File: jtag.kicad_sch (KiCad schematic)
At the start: 50 parts, among them J3 USB_C_Receptacle, J4 Conn_01x02_Male, J5 3220-10-0100-00, U10 NTB0104BQ,115, U13 NTB0104BQ,115, U17 93C56, U2 FT2232HL-REEL, Y2 12MHz

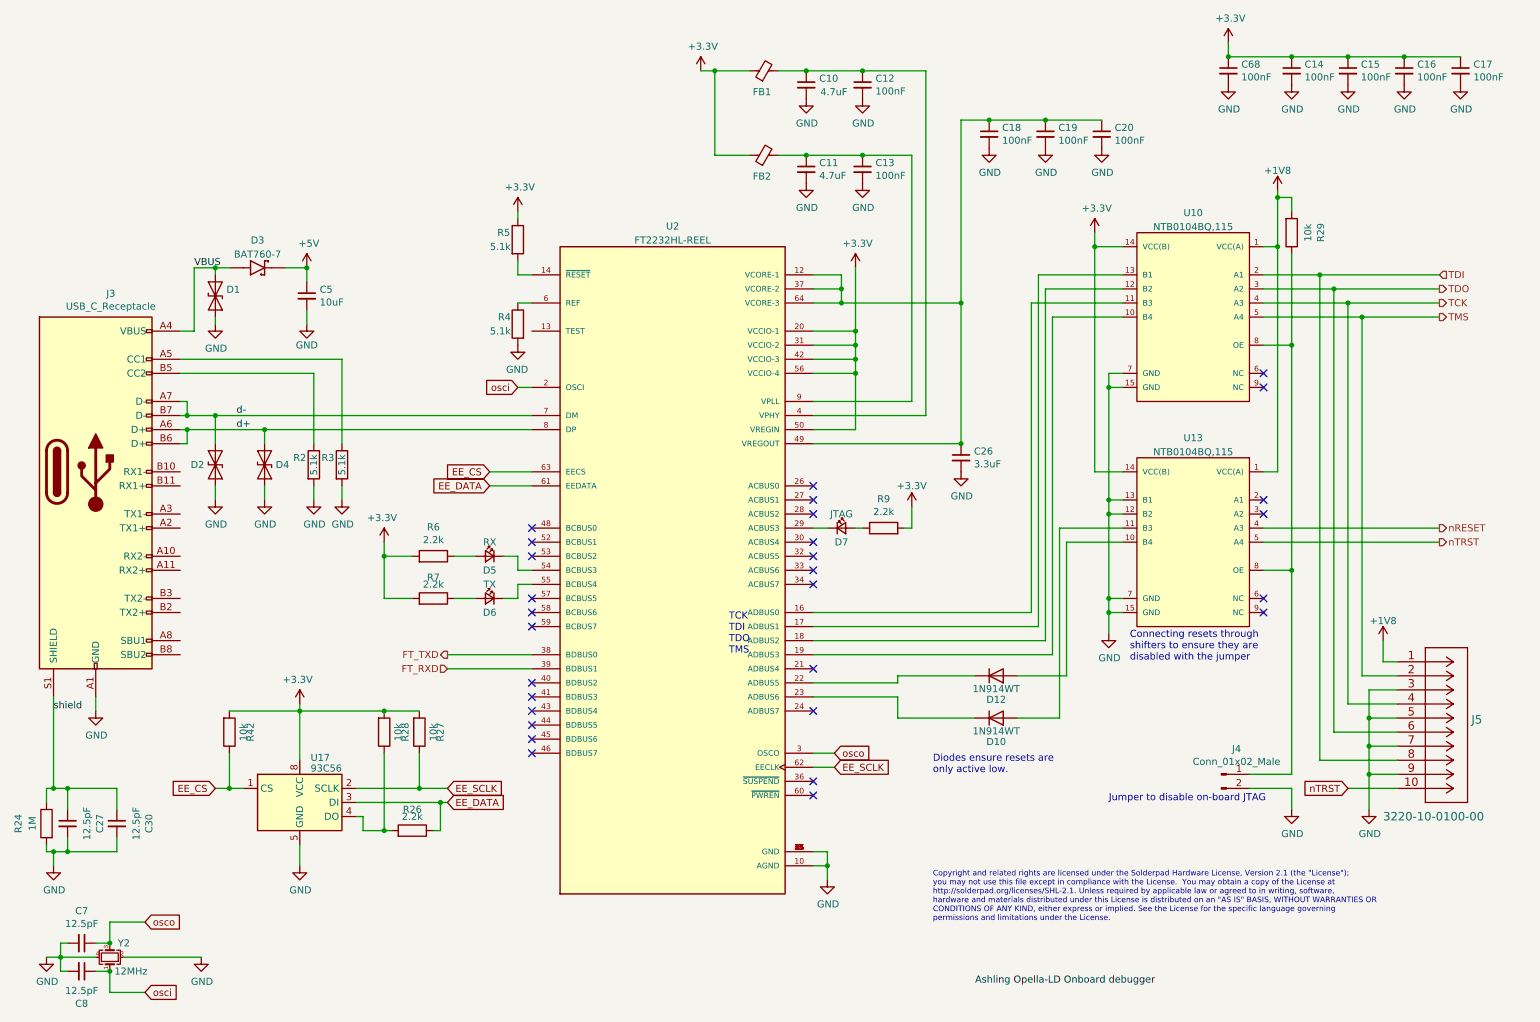
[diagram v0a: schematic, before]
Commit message: updated footprints, added the barrel power connector and test points
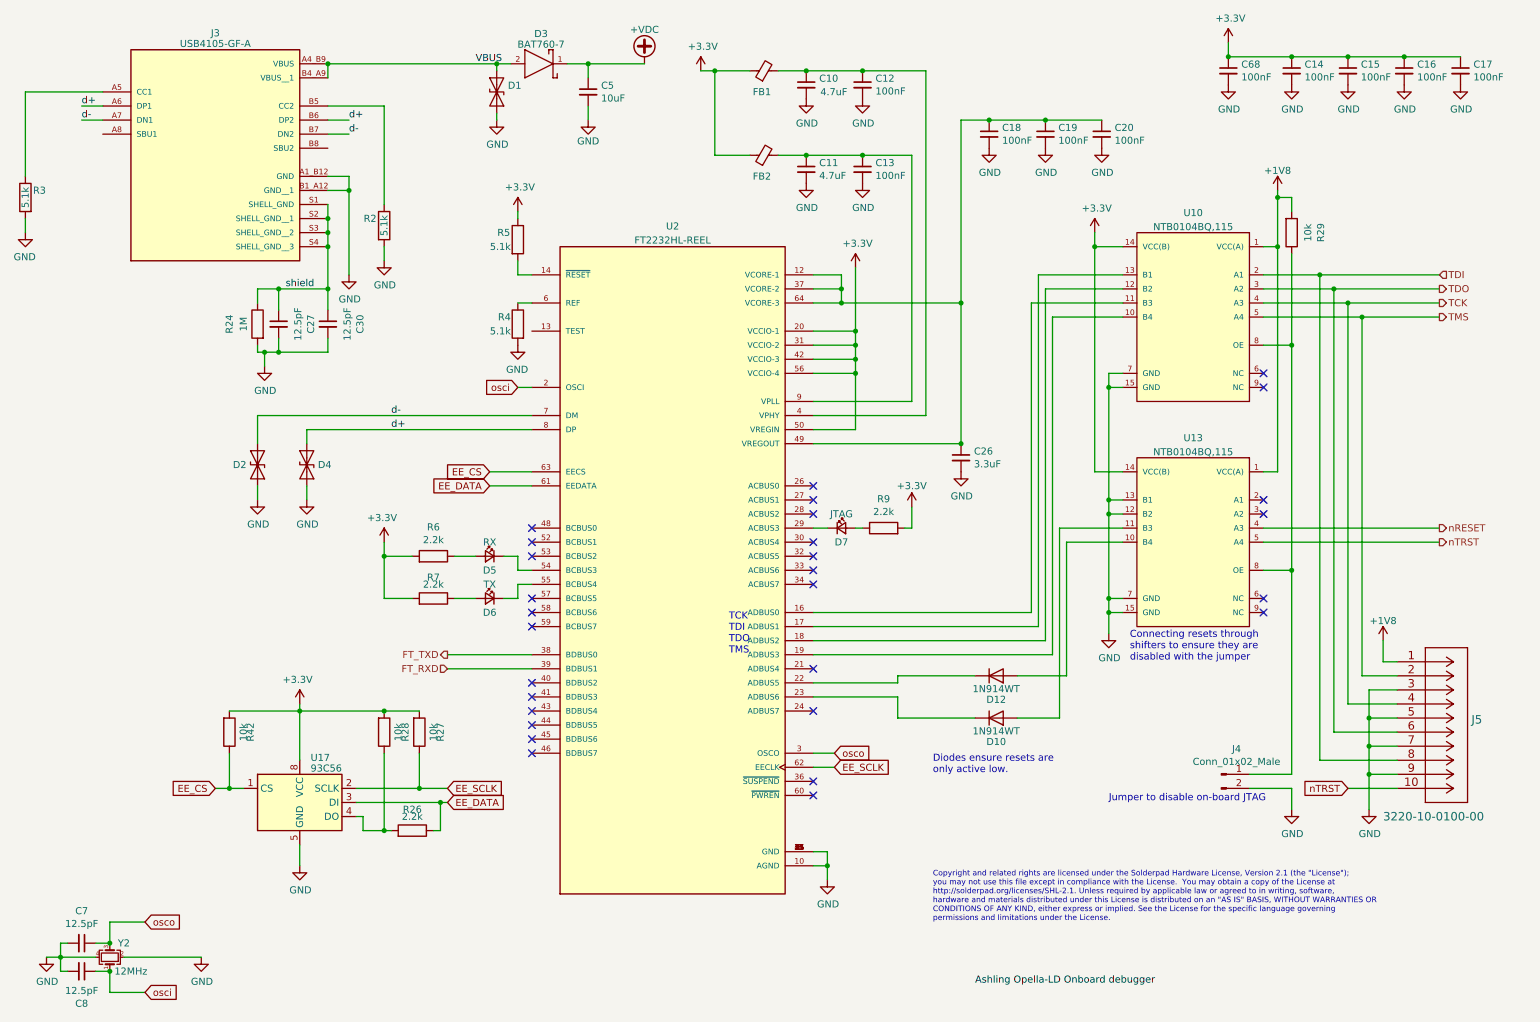
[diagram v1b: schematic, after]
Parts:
- removed D3: BAT760-7, Diode_SMD:SOD2513X120N, symbol bat760:BAT760-7
- removed J3: USB_C_Receptacle, Connector_USB:USB_C_Receptacle_Amphenol_12401610E4-2A, symbol Connector:USB_C_Receptacle
- added D3: BAT760-7, diode:Diodes-SOD323-03_2017-0-0, symbol diode:BAT760-7
- added J3: USB4105-GF-A, GCT_USB4105-GF-A, symbol usb:USB4105-GF-A
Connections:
- net GND: now also J3.A1_B12 (GND), J3.B1_A12 (GND__1)
- net VBUS: now also D3.2 (ANODE), J3.A4_B9 (VBUS), J3.B4_A9 (VBUS__1)
- net d+: now also J3.A6 (DP1), J3.B6 (DP2)
- net d-: now also J3.A7 (DN1), J3.B7 (DN2)
- net shield: now also J3.S1 (SHELL_GND), J3.S2 (SHELL_GND__1), J3.S3 (SHELL_GND__2), J3.S4 (SHELL_GND__3)
- net at R3.1: now also J3.A5 (CC1)
- net at R2.1: now also J3.B5 (CC2)
- net +5V renamed +VDC
- net +VDC: now also D3.1 (CATHODE)
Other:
- moved on the sheet: C27, C30, C5, D1, D2, D4, R2, R24, R3
